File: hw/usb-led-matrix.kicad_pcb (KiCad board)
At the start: 2 copper layers, 76 parts, among them J2 Conn_ARM_JTAG_SWD_10, U1 AP1117-33, U2 stm32g473, U3 74LVT244A

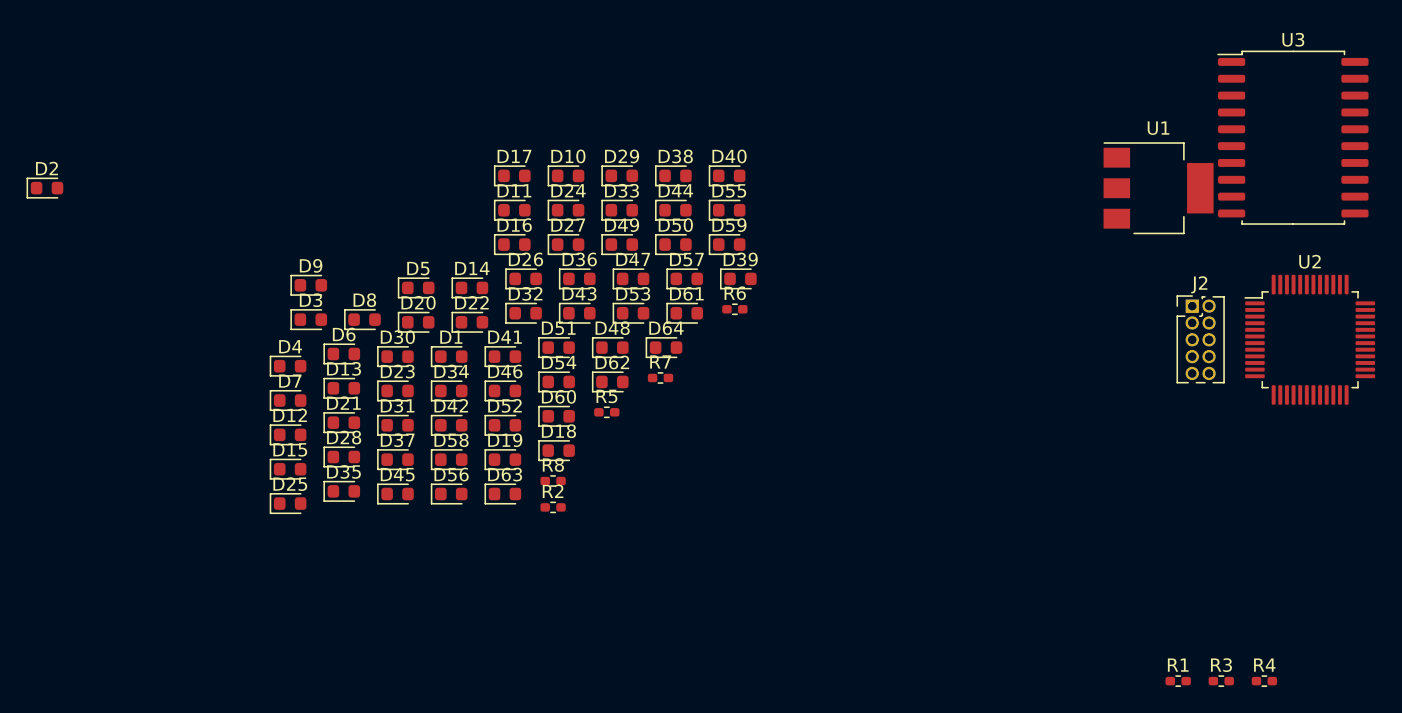
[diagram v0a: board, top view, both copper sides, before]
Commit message: Updates
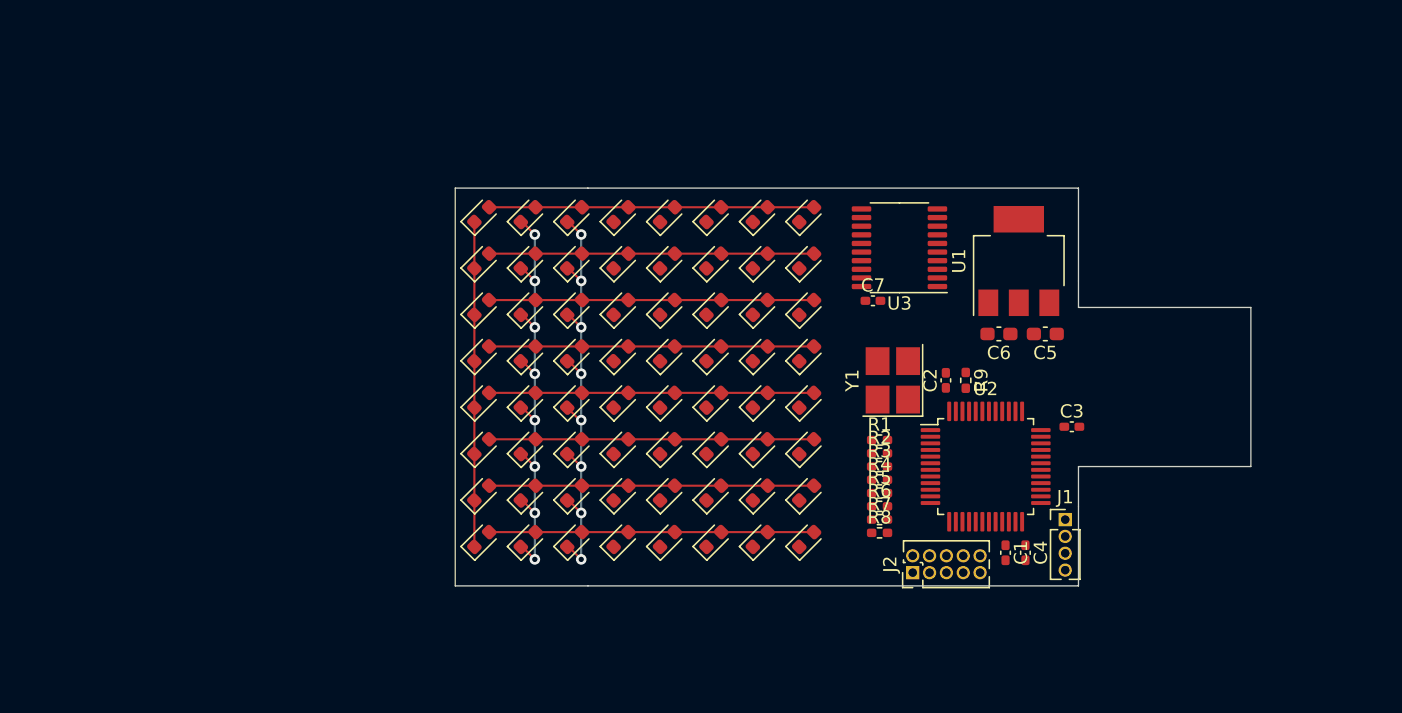
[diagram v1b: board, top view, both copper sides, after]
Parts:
- added C1: C, Capacitor_SMD:C_0402_1005Metric_Pad0.74x0.62mm_HandSolder, F.Cu at (181.5, 107.5)
- added C2: C, Capacitor_SMD:C_0402_1005Metric_Pad0.74x0.62mm_HandSolder, F.Cu at (177.0, 94.5)
- added C3: C, Capacitor_SMD:C_0402_1005Metric_Pad0.74x0.62mm_HandSolder, F.Cu at (186.5, 98.0)
- added C4: C, Capacitor_SMD:C_0402_1005Metric_Pad0.74x0.62mm_HandSolder, F.Cu at (183.0, 107.5)
- added C5: C, Capacitor_SMD:C_0603_1608Metric_Pad1.08x0.95mm_HandSolder, F.Cu at (184.5, 91.0)
- added C6: C, Capacitor_SMD:C_0603_1608Metric_Pad1.08x0.95mm_HandSolder, F.Cu at (181.0, 91.0)
- added C7: C, Capacitor_SMD:C_0402_1005Metric_Pad0.74x0.62mm_HandSolder, F.Cu at (171.5, 88.5)
- added J1: Conn_01x04_Male, Connector_PinHeader_1.27mm:PinHeader_1x04_P1.27mm_Vertical, F.Cu at (186.0, 105.0)
- added R9: R, Resistor_SMD:R_0402_1005Metric_Pad0.72x0.64mm_HandSolder, F.Cu at (178.5, 94.5)
- added Y1: Crystal_GND23, Crystal:Crystal_SMD_3225-4Pin_3.2x2.5mm_HandSoldering, F.Cu at (173.0, 94.5)
- U3: value 74LVT244A -> 74LVT245; footprint Package_SO:SOIC-20W_7.5x12.8mm_P1.27mm -> Package_SO:TSSOP-20_4.4x6.5mm_P0.65mm
- moved D2 33.2 mm to (142.0, 85.5), turned to 45 degrees
- moved D25 33.1 mm to (152.5, 82.0), turned to 45 degrees
- moved R4 32.8 mm to (172.0, 102.0)
- moved U3 30.8 mm to (173.5, 84.5), turned to 180 degrees
- moved D58 30.7 mm to (166.5, 85.5), turned to 45 degrees
- moved R3 30.4 mm to (172.0, 101.0)
- moved J2 29.1 mm to (174.5, 109.0), turned to 90 degrees
- moved R1 28.9 mm to (172.0, 99.0)
- moved D35 28.1 mm to (156.0, 89.0), turned to 45 degrees
- moved D40 27.8 mm to (156.0, 106.5), turned to 45 degrees
- moved U2 26.3 mm to (180.0, 101.0)
- moved R2 25.0 mm to (172.0, 100.0)
- moved R8 24.9 mm to (172.0, 106.0)
- moved D45 24.9 mm to (159.5, 96.0), turned to 45 degrees
- moved D24 24.8 mm to (149.0, 106.5), turned to 45 degrees
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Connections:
- J2 pad 1: Net-(J2-Pad1) -> /VDD
- J2 pad 10: Net-(J2-Pad10) -> /NRST
- J2 pad 2: Net-(J2-Pad2) -> /SWDIO
- J2 pad 3: Net-(J2-Pad3) -> GND
- J2 pad 4: Net-(J2-Pad4) -> /SWCLK
- J2 pad 5: Net-(J2-Pad3) -> GND
- J2 pad 9: Net-(J2-Pad9) -> GND
- U1 pad 1: Net-(U1-Pad1) -> GND
- U1 pad 2: Net-(U1-Pad2) -> /VDD
- U2 pad 19: Net-(U2-Pad19) -> GND
- U2 pad 21: Net-(U2-Pad21) -> /VDD
- U2 pad 23: Net-(U2-Pad23) -> GND
- U2 pad 24: Net-(U2-Pad24) -> /VDD
- U2 pad 35: Net-(U2-Pad35) -> GND
- U2 pad 36: Net-(U2-Pad36) -> /VDD
- U2 pad 45: Net-(U2-Pad45) -> /BOOT0
- U2 pad 47: Net-(U2-Pad47) -> GND
- U2 pad 48: Net-(U2-Pad48) -> /VDD
- U2 pad 7: Net-(U2-Pad7) -> /NRST
- U3 pad 10: Net-(U3-Pad10) -> GND
- U3 pad 11: /COL1 -> Net-(D1-Pad1)
- U3 pad 12: Net-(D33-Pad1) -> Net-(D10-Pad1)
- U3 pad 13: /COL2 -> Net-(D17-Pad1)
- U3 pad 14: Net-(D41-Pad1) -> Net-(D25-Pad1)
- U3 pad 15: /COL3 -> Net-(D33-Pad1)
- U3 pad 16: Net-(D49-Pad1) -> Net-(D41-Pad1)
- U3 pad 17: /COL4 -> Net-(D49-Pad1)
- U3 pad 20: Net-(U3-Pad20) -> /VDD
- U3 pad 3: Net-(D25-Pad1) -> /COL7
- U3 pad 4: /COL7 -> /COL6
- U3 pad 5: Net-(D17-Pad1) -> /COL5
- U3 pad 6: /COL6 -> /COL4
- U3 pad 7: Net-(D10-Pad1) -> /COL3
- U3 pad 8: /COL5 -> /COL2
- U3 pad 9: Net-(D1-Pad1) -> /COL1
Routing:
- net Net-(D17-Pad1): track 0.00 -> 36.1 mm, vias 0 -> 8
- net Net-(D10-Pad1): track 0.00 -> 36.1 mm, vias 0 -> 8
- net Net-(D16-Pad2): track 0.00 -> 24.5 mm
- net Net-(D15-Pad2): track 0.00 -> 24.5 mm
- net Net-(D14-Pad2): track 0.00 -> 24.5 mm
- net Net-(D13-Pad2): track 0.00 -> 24.5 mm
- net Net-(D12-Pad2): track 0.00 -> 24.5 mm
- net Net-(D11-Pad2): track 0.00 -> 24.5 mm
- net Net-(D10-Pad2): track 0.00 -> 24.5 mm
- net Net-(D1-Pad2): track 0.00 -> 24.5 mm
- net Net-(D1-Pad1): track 0.00 -> 24.5 mm
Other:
- board outline added: 60 x 30 mm
- net class Default: trace_width 0.25 -> 0.16
- net class Power added: clearance 0.2, trace_width 0.3, via_dia 0.8, via_drill 0.4
- rule trace_min: 0.2 -> 0.15

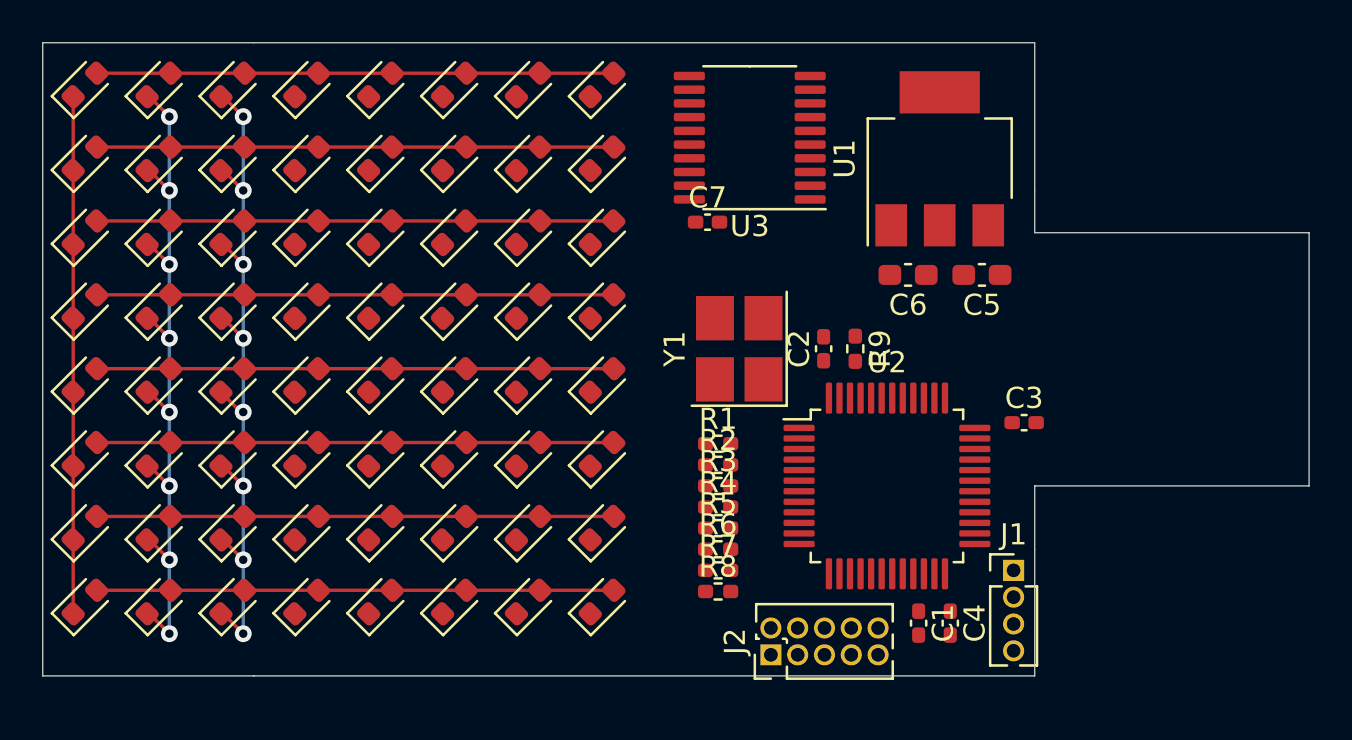
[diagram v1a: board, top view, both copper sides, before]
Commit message: Work
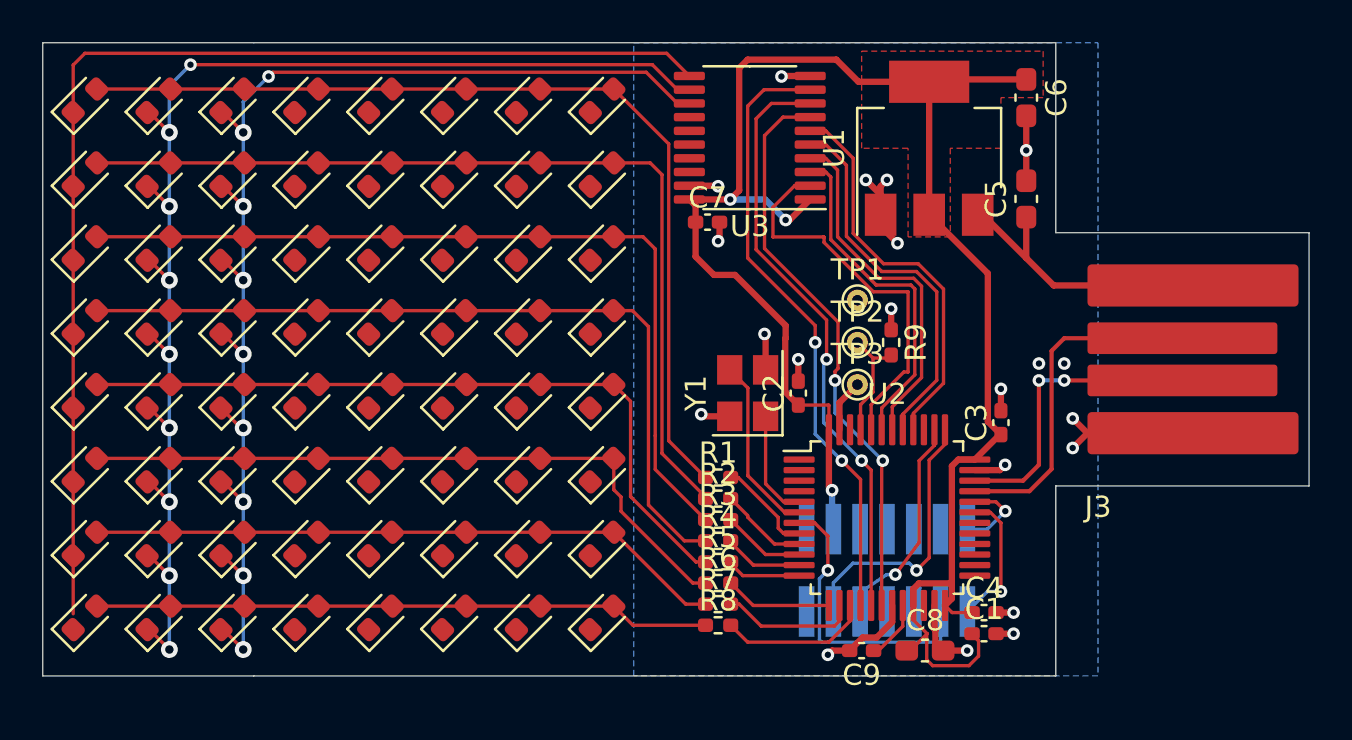
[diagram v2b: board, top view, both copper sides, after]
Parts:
- removed J1: Conn_01x04_Male, Connector_PinHeader_1.27mm:PinHeader_1x04_P1.27mm_Vertical
- added C8: C, Capacitor_SMD:C_0603_1608Metric_Pad1.08x0.95mm_HandSolder, F.Cu at (181.8, 108.8)
- added C9: C, Capacitor_SMD:C_0402_1005Metric_Pad0.74x0.62mm_HandSolder, F.Cu at (178.8, 108.8)
- added J3: USB_A, usb-board-edge:usb-a-board-edge, F.Cu at (195.0, 95.0)
- added TP1: TestPoint, TestPoint:TestPoint_THTPad_D1.0mm_Drill0.5mm, F.Cu at (178.6, 92.2)
- added TP2: TestPoint, TestPoint:TestPoint_THTPad_D1.0mm_Drill0.5mm, F.Cu at (178.6, 94.2)
- added TP3: TestPoint, TestPoint:TestPoint_THTPad_D1.0mm_Drill0.5mm, F.Cu at (178.6, 96.2)
- J2: value Conn_ARM_JTAG_SWD_10 -> Conn_ST_STDC14; footprint Connector_PinHeader_1.27mm:PinHeader_2x05_P1.27mm_Vertical -> Connector_PinHeader_1.27mm:PinHeader_2x07_P1.27mm_Vertical_SMD; moved to B.Cu
- U2: value stm32g473 -> STM32G473CET6
- Y1: value Crystal_GND23 -> Crystal_GND24; footprint Crystal:Crystal_SMD_3225-4Pin_3.2x2.5mm_HandSoldering -> Crystal:Crystal_SMD_3225-4Pin_3.2x2.5mm
- moved C6 10.1 mm to (186.6, 82.6), turned to 270 degrees
- moved J2 6.80 mm to (180.0, 105.0), turned to 270 degrees
- moved C5 4.17 mm to (186.6, 87.4), turned to 90 degrees
- moved C1 3.14 mm to (184.6, 108.0), turned to 0 degrees
- moved C2 2.42 mm to (175.8, 96.6)
- moved Y1 2.14 mm to (173.4, 96.6)
- moved R9 1.73 mm to (180.2, 94.2)
- moved C4 1.68 mm to (184.6, 107.0), turned to 0 degrees
- moved R1 1.60 mm to (172.0, 100.6)
- moved R2 1.60 mm to (172.0, 101.6)
- moved R3 1.60 mm to (172.0, 102.6)
- moved R4 1.60 mm to (172.0, 103.6)
- moved R5 1.60 mm to (172.0, 104.6)
- moved R6 1.60 mm to (172.0, 105.6)
- moved R7 1.60 mm to (172.0, 106.6)
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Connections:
- net Net-(C5-Pad1) renamed /VBUS
- J2 pad 1: /VDD -> Net-(J2-Pad1)
- J2 pad 10: /NRST -> Net-(J2-Pad10)
- J2 pad 2: /SWDIO -> Net-(J2-Pad2)
- J2 pad 3: GND -> /VDD
- J2 pad 4: /SWCLK -> /SWDIO
- J2 pad 6: Net-(J2-Pad6) -> /SWCLK
- J2 pad 7: Net-(J2-Pad7) -> GND
- J2 pad 9: GND -> Net-(J2-Pad9)
- R9 pad 1: Net-(R9-Pad1) -> GND
- U2 pad 31: Net-(U2-Pad31) -> /TX
- U2 pad 32: Net-(U2-Pad32) -> /RX
- U3 pad 1: Net-(U3-Pad1) -> /VDD
- U3 pad 19: Net-(U3-Pad19) -> GND
- Y1 pad 2: Net-(Y1-Pad2) -> GND
- Y1 pad 3: Net-(Y1-Pad3) -> Net-(U2-Pad6)
- Y1 pad 4: Net-(U2-Pad6) -> GND
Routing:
- net /VDD: track 0.00 -> 87.2 mm, vias 0 -> 3
- net GND: track 0.00 -> 38.9 mm, vias 0 -> 21
- net Net-(D1-Pad1): track 24.5 -> 55.9 mm
- net /COL1: track 0.00 -> 29.2 mm, vias 0 -> 2
- net /COL2: track 0.00 -> 28.3 mm, vias 0 -> 2
- net Net-(D10-Pad1): track 36.1 -> 63.8 mm, vias 8 -> 9
- net /COL3: track 0.00 -> 27.2 mm, vias 0 -> 2
- net Net-(D17-Pad1): track 36.1 -> 59.9 mm, vias 8 -> 9
- net Net-(D1-Pad2): track 24.5 -> 44.7 mm
- net /COL4: track 0.00 -> 18.8 mm
- net Net-(D10-Pad2): track 24.5 -> 43.2 mm
- net /COL8: track 0.00 -> 18.6 mm
- net /COL5: track 0.00 -> 18.1 mm
- net /COL6: track 0.00 -> 17.0 mm
- net /COL7: track 0.00 -> 16.3 mm
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- added copper zone on F.Cu, net /VDD
- added copper zone on B.Cu, net GND
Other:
- outline, holes or cut-outs redrawn
- net class Default: clearance 0.2 -> 0.16; via_dia 0.8 -> 0.6; via_drill 0.4 -> 0.3
- net class Power: clearance 0.2 -> 0.16; via_dia 0.8 -> 0.6; via_drill 0.4 -> 0.3
- net class USB added: clearance 0.2, trace_width 0.2, via_dia 0.6, via_drill 0.3
- rule trace_clearance: 0.2 -> 0.16
- rule trace_min: 0.15 -> 0.1
- rule via_min_size: 0.4 -> 0.6
